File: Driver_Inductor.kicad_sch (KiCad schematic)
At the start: 6 parts, among them J1 Control_A, J2 DC+, J3 DC-, J4 OUT1, J5 OUT2

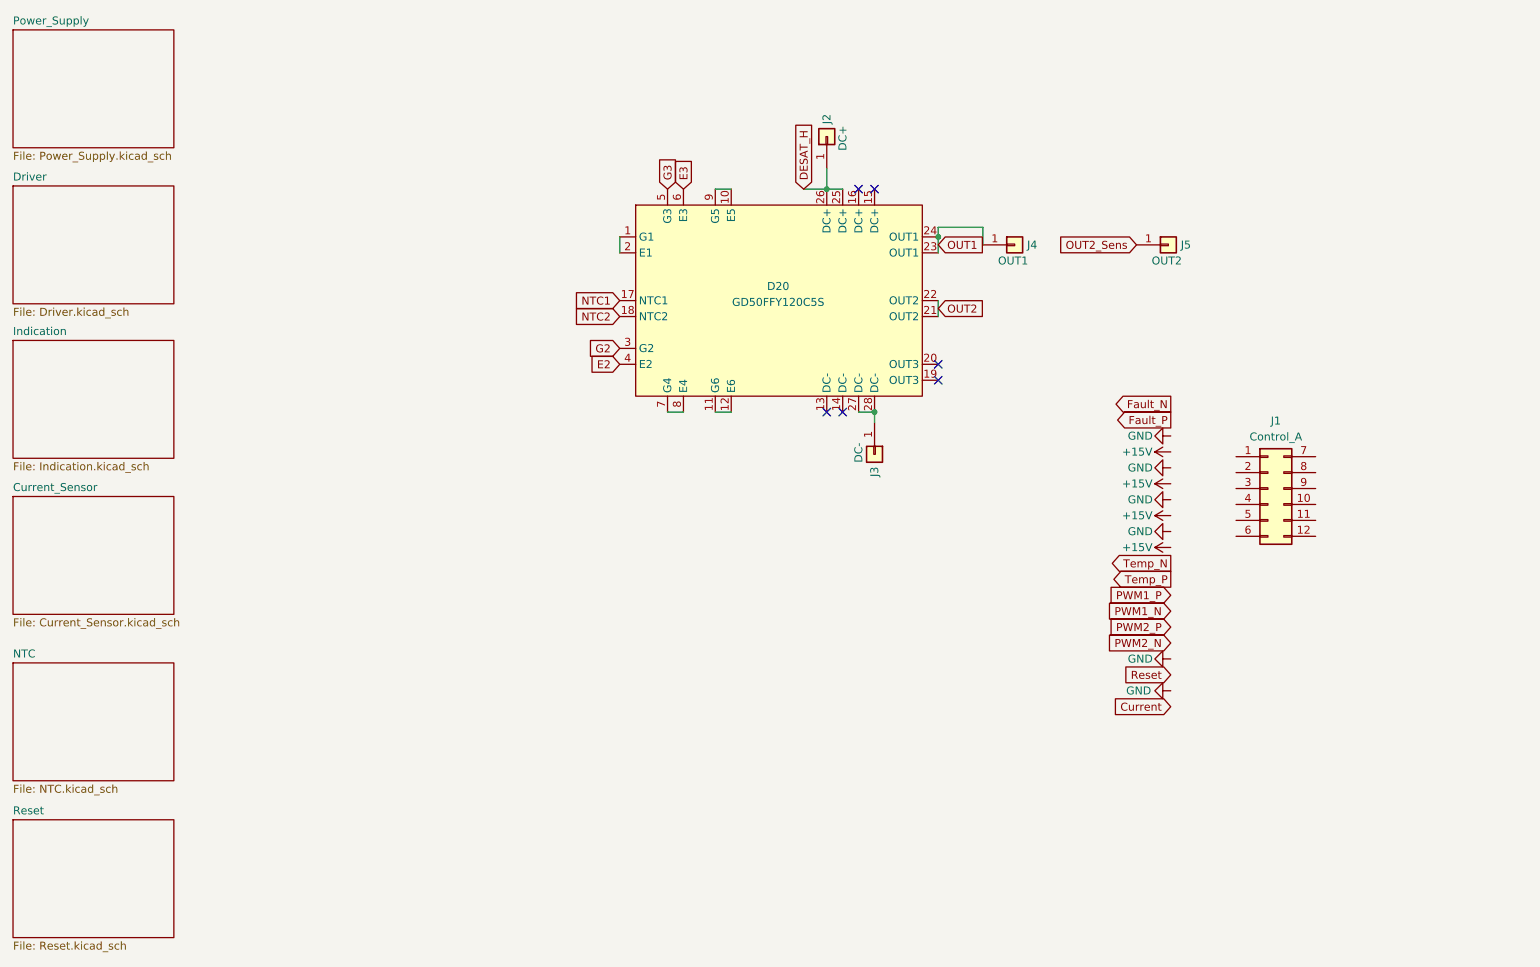
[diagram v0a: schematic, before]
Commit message: Развел все дорожки
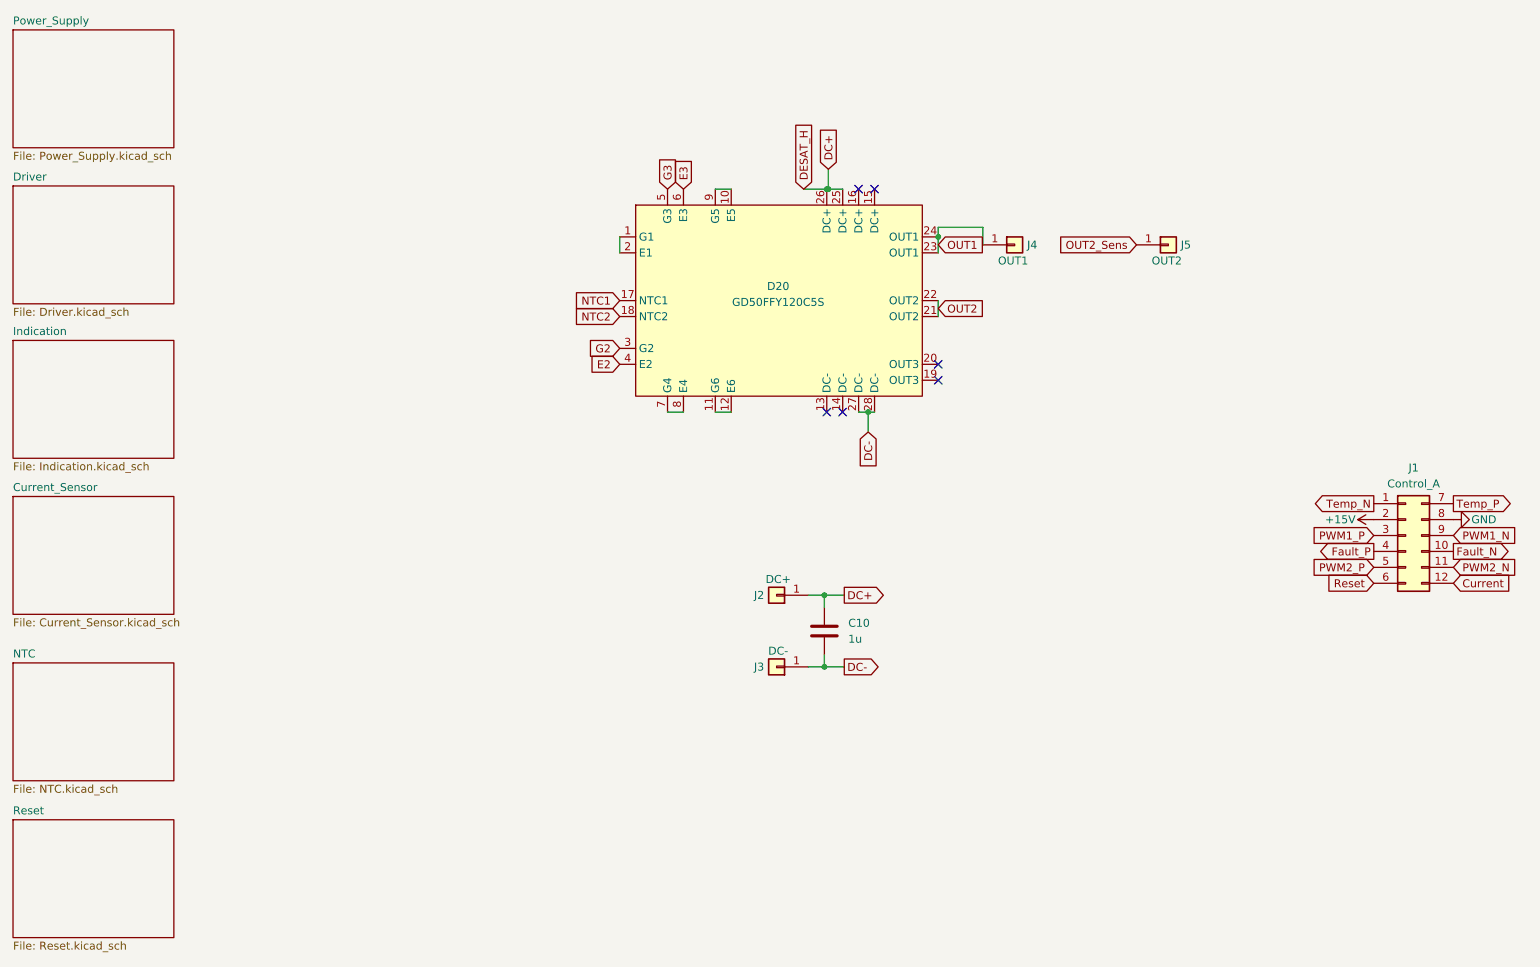
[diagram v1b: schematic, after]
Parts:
- added C10: 1u, Capacitor_THT:C_Rect_L31.5mm_W13.0mm_P27.50mm_MKS4, symbol Device:C
- J2, J3, J4, J5: footprint Connector_Power:M5 -> Connector_My:Bush_M4
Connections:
- net +15V: now also J1.2 (Pin_2)
- net Current: now also J1.12 (Pin_12)
- net Fault_N: now also J1.10 (Pin_10)
- net Fault_P: now also J1.4 (Pin_4)
- net GND: now also J1.8 (Pin_8)
- net PWM1_N: now also J1.9 (Pin_9)
- net PWM1_P: now also J1.3 (Pin_3)
- net PWM2_N: now also J1.11 (Pin_11)
- net PWM2_P: now also J1.5 (Pin_5)
- net Reset: now also J1.6 (Pin_6)
- net Temp_N: now also J1.1 (Pin_1)
- net Temp_P: now also J1.7 (Pin_7)
- net DC-: now reaches D20.27 (DC-), D20.28 (DC-), J3.1 (Pin_1)
- net DC-: now also C10.2
- net DESAT_H renamed DC+
- net DC+: now also C10.1
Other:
- moved on the sheet: J1, J2, J3
